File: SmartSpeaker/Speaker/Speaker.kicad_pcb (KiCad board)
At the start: 2 copper layers, 6.2 x 5.8 mm, 34 parts, among them J103 Screw_Terminal_01x02, J3 54-00166, Q1 DMG2305UX-13, U1 LM384, U2 LTC1655LCN8, U3 LM2675N-5, U4 LM4040LP-3

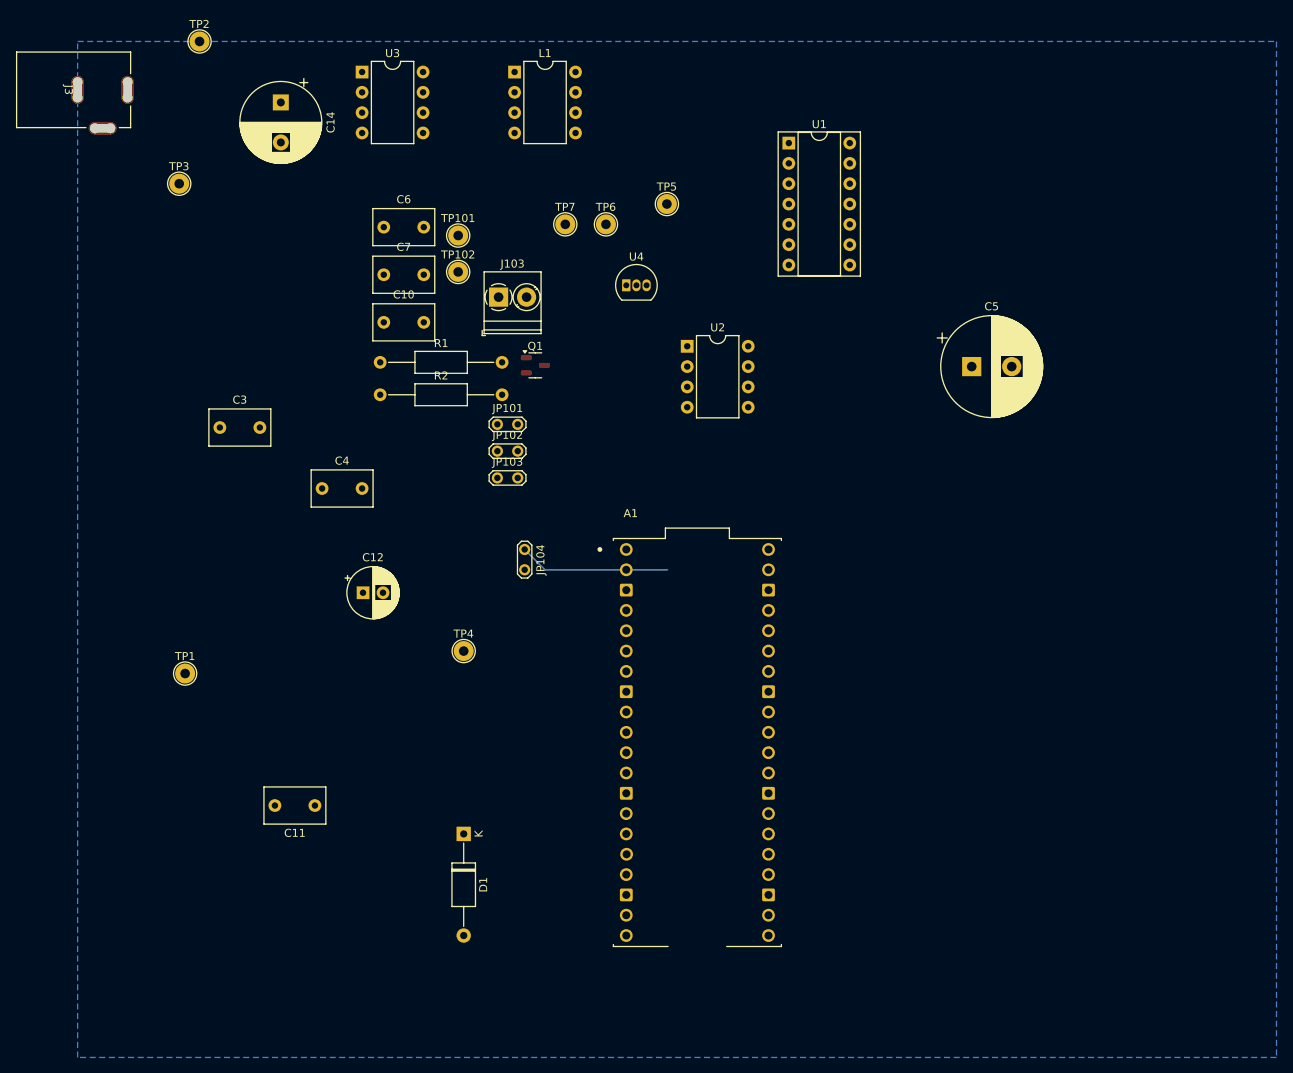
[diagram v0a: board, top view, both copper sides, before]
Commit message: PCB progress
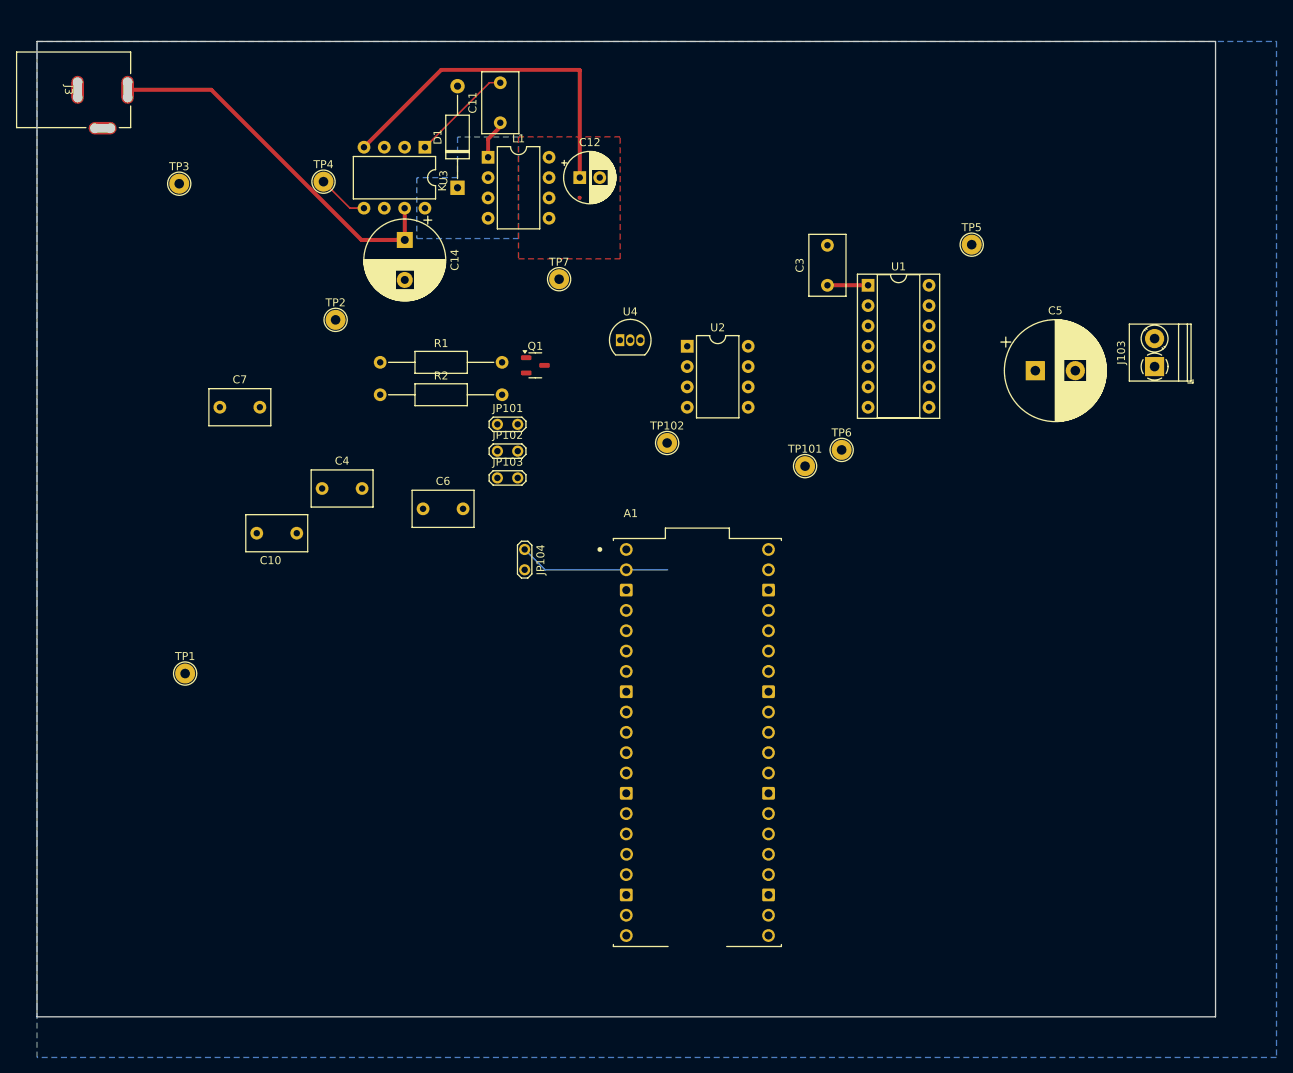
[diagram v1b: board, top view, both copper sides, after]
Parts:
- moved C11 88.4 mm to (93.5, 35.6), turned to 90 degrees
- moved J103 82.5 mm to (175.3, 66.0), turned to 90 degrees
- moved D1 80.8 mm to (88.1, 43.7), turned to 90 degrees
- moved C3 78.0 mm to (134.4, 55.9), turned to 90 degrees
- moved TP4 61.2 mm to (71.4, 42.9)
- moved C12 58.5 mm to (103.4, 42.4)
- moved TP101 52.1 mm to (131.6, 78.5)
- moved TP6 40.8 mm to (136.1, 76.5)
- moved TP2 38.7 mm to (72.9, 60.2)
- moved TP5 38.4 mm to (152.4, 50.8)
- moved C6 35.6 mm to (83.8, 83.8)
- moved TP102 33.8 mm to (114.3, 75.6)
- moved C10 30.8 mm to (63.0, 86.9)
- moved C7 26.3 mm to (58.4, 71.1)
- moved C14 23.1 mm to (81.5, 50.2)
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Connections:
- net Net-(C5-Pad1) renamed /AudioOut
- net Net-(J103-Pin_1) renamed /SpeakerOut
- C11 pad 1: Net-(D1-K) -> /Power_converter/VSwitch
- D1 pad 1: Net-(D1-K) -> /Power_converter/VSwitch
- L1 pad 1: Net-(D1-K) -> /Power_converter/VSwitch
- L1 pad 2: /Power_converter/5VOut -> /Power_converter/VSwitch
- L1 pad 3: (no net) -> /Power_converter/VSwitch
- L1 pad 4: (no net) -> /Power_converter/VSwitch
- L1 pad 5: (no net) -> /Power_converter/5VOut
- L1 pad 6: (no net) -> /Power_converter/5VOut
- L1 pad 7: (no net) -> /Power_converter/5VOut
- L1 pad 8: (no net) -> /Power_converter/5VOut
- U3 pad 8: Net-(D1-K) -> /Power_converter/VSwitch
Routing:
- net /Power_converter/VoltageIn: track 18.9 -> 64.6 mm
- net /Power_converter/5VOut: track 0.00 -> 44.5 mm
- net Net-(U3-CB): track 0.00 -> 12.8 mm
- net Net-(U3-ON/~{OFF}): track 0.00 -> 6.43 mm
- net /Power_converter/VSwitch: track 0.00 -> 5.16 mm
- net Net-(U1-BYPASS): track 0.00 -> 5.08 mm
- net /SpeakerOut: track 0.00 -> 1.84 mm
- added copper zone on F.Cu, net /Power_converter/5VOut
- added copper zone on B.Cu, net /Power_converter/VSwitch
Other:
- board size 6.2 x 5.8 mm -> 147.3 x 121.9 mm
